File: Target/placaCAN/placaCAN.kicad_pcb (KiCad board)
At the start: 2 copper layers, 5 parts, among them J1 Can1, J2 Can2, j3 a PC

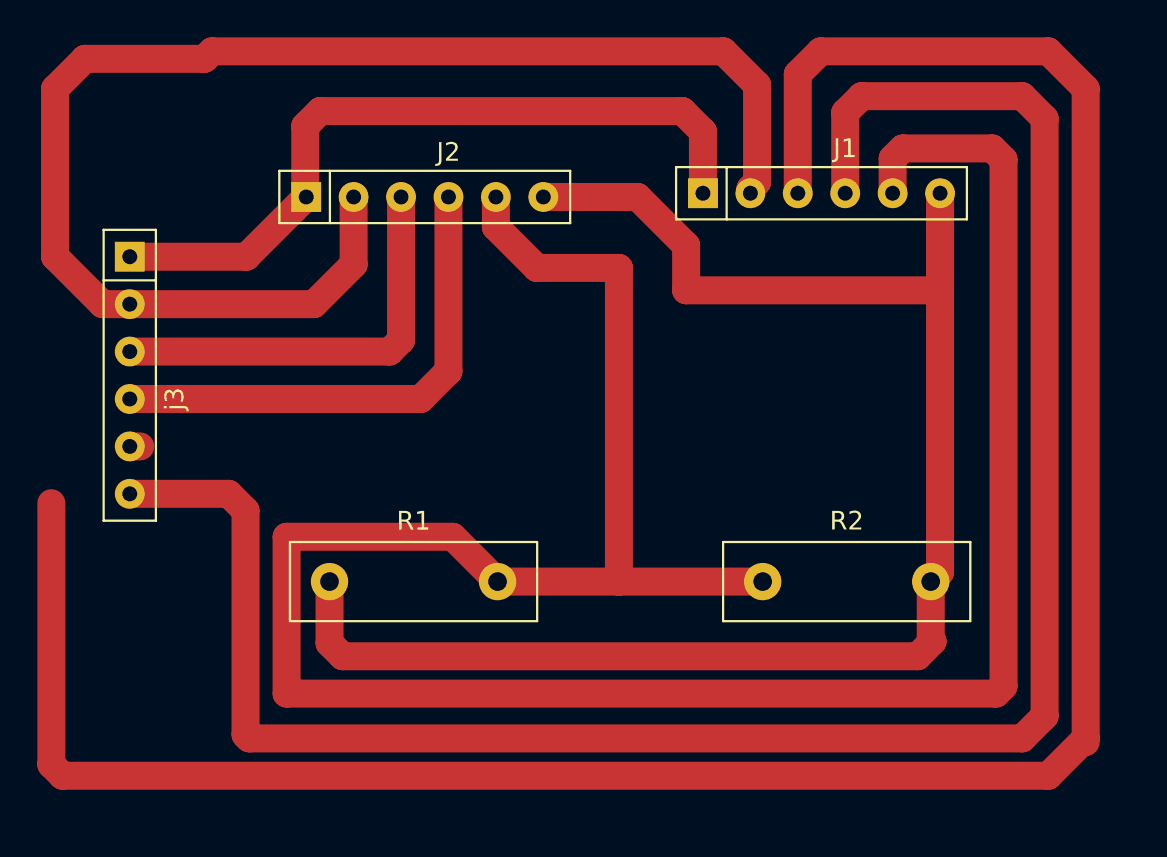
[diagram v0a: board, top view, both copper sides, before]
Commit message: actualizo
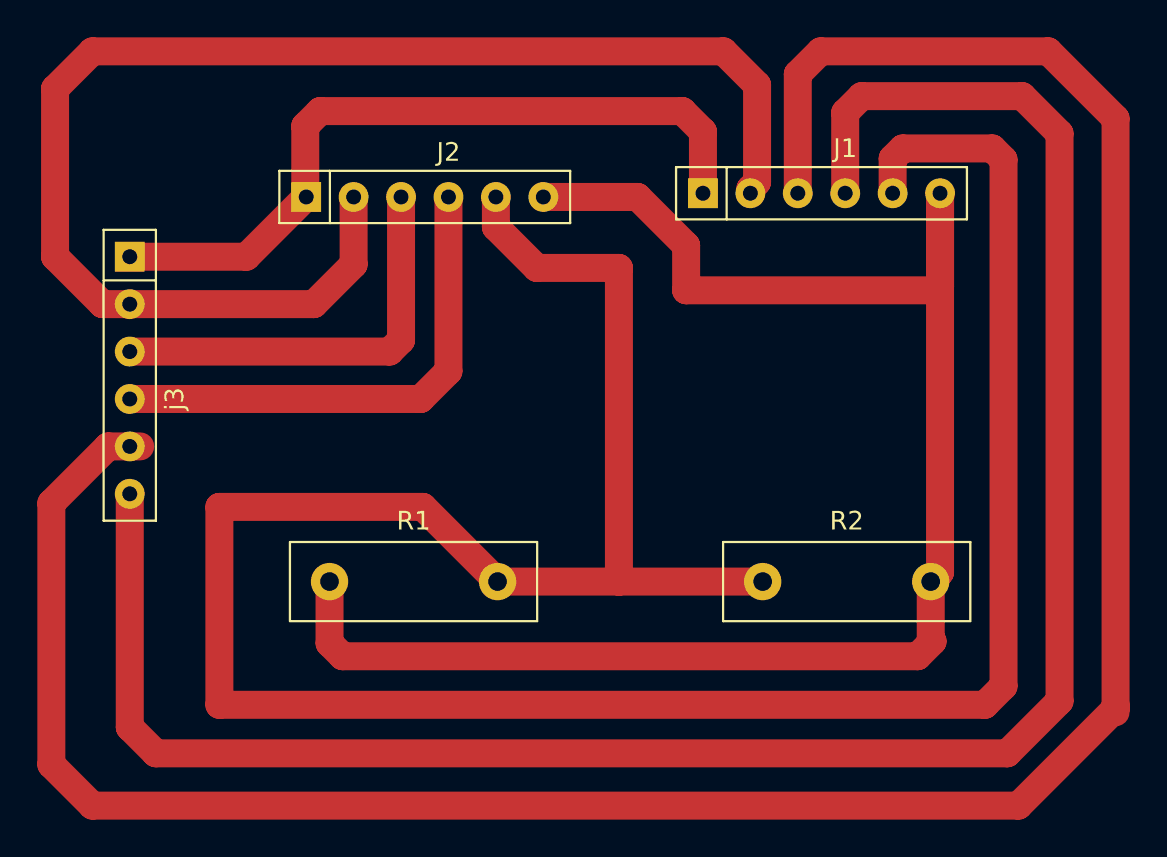
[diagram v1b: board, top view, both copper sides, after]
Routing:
- net Net-(J1-Pad5): track 135.8 -> 146.2 mm
- net Net-(J1-Pad3): track 129.2 -> 137.5 mm
- net Net-(J1-Pad4): track 109.8 -> 111.4 mm
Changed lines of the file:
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@@
   (segment (start 122.2 69.95) (end 122.25 70) (width 1.5) (layer "F.Cu") (net 1))
   (segment (start 124.79 73.61) (end 124.79 70) (width 1.5) (layer "F.Cu") (net 2))
-  (segment (start 117.2 62.2) (end 144.6 62.2) (width 1.5) (layer "F.Cu") (net 2))
-  (segment (start 146.4 69.2) (end 146.04 69.56) (width 1.5) (layer "F.Cu") (net 2))
+  (segment (start 144.6 62.2) (end 146.4 64) (width 1.5) (layer "F.Cu") (net 2))
   (segment (start 112.8 75.74) (end 111.34 75.74) (width 1.5) (layer "F.Cu") (net 2))
   (segment (start 122.66 75.74) (end 124.79 73.61) (width 1.5) (layer "F.Cu") (net 2))
   (segment (start 112.8 75.74) (end 122.66 75.74) (width 1.5) (layer "F.Cu") (net 2))
-  (segment (start 144.6 62.2) (end 146.4 64) (width 1.5) (layer "F.Cu") (net 2))
-  (segment (start 108.8 64.2) (end 110.4 62.6) (width 1.5) (layer "F.Cu") (net 2))
-  (segment (start 116.8 62.6) (end 117.2 62.2) (width 1.5) (layer "F.Cu") (net 2))
+  (segment (start 111.34 75.74) (end 108.8 73.2) (width 1.5) (layer "F.Cu") (net 2))
+  (segment (start 108.8 64.2) (end 110.8 62.2) (width 1.5) (layer "F.Cu") (net 2))
+  (segment (start 146.4 69.2) (end 146.04 69.56) (width 1.5) (layer "F.Cu") (net 2))
+  (segment (start 146.4 64) (end 146.4 69.2) (width 1.5) (layer "F.Cu") (net 2))
   (segment (start 108.8 73.2) (end 108.8 64.2) (width 1.5) (layer "F.Cu") (net 2))
-  (segment (start 111.34 75.74) (end 108.8 73.2) (width 1.5) (layer "F.Cu") (net 2))
-  (segment (start 146.4 64) (end 146.4 69.2) (width 1.5) (layer "F.Cu") (net 2))
   (segment (start 146.04 69.56) (end 146.04 69.8) (width 1.5) (layer "F.Cu") (net 2))
-  (segment (start 110.4 62.6) (end 116.8 62.6) (width 1.5) (layer "F.Cu") (net 2))
-  (segment (start 149.8 62.2) (end 162 62.2) (width 1.5) (layer "F.Cu") (net 3))
+  (segment (start 110.8 62.2) (end 144.6 62.2) (width 1.5) (layer "F.Cu") (net 2))
+  (segment (start 165.6 97.2) (end 165.6 97.4) (width 1.5) (layer "F.Cu") (net 3))
   (segment (start 148.58 63.42) (end 149.8 62.2) (width 1.5) (layer "F.Cu") (net 3))
   (segment (start 113.36 83.36) (end 112.8 83.36) (width 1.5) (layer "F.Cu") (net 3))
-  (segment (start 162 62.2) (end 164 64.2) (width 1.5) (layer "F.Cu") (net 3))
-  (segment (start 164 64.2) (end 164 99.2) (width 1.5) (layer "F.Cu") (net 3))
+  (segment (start 160.4 102.6) (end 110.8 102.6) (width 1.5) (layer "F.Cu") (net 3))
+  (segment (start 165.6 65.8) (end 165.6 97.6) (width 1.5) (layer "F.Cu") (net 3))
+  (segment (start 110.8 102.6) (end 108.6 100.4) (width 1.5) (layer "F.Cu") (net 3))
+  (segment (start 148.58 69.8) (end 148.58 63.42) (width 1.5) (layer "F.Cu") (net 3))
   (segment (start 108.6 100.4) (end 108.6 86.4) (width 1.5) (layer "F.Cu") (net 3))
-  (segment (start 164 99) (end 162 101) (width 1.5) (layer "F.Cu") (net 3))
-  (segment (start 109.2 101) (end 108.6 100.4) (width 1.5) (layer "F.Cu") (net 3))
-  (segment (start 162 101) (end 109.2 101) (width 1.5) (layer "F.Cu") (net 3))
-  (segment (start 148.58 69.8) (end 148.58 63.42) (width 1.5) (layer "F.Cu") (net 3))
-  (segment (start 118.1 85.9) (end 119 86.8) (width 1.5) (layer "F.Cu") (net 4))
-  (segment (start 161.8 97.8) (end 160.6 99) (width 1.5) (layer "F.Cu") (net 4))
-  (segment (start 160.6 99) (end 119.2 99) (width 1.5) (layer "F.Cu") (net 4))
+  (segment (start 111.64 83.36) (end 112.8 83.36) (width 1.5) (layer "F.Cu") (net 3))
+  (segment (start 165.6 97.4) (end 160.4 102.6) (width 1.5) (layer "F.Cu") (net 3))
+  (segment (start 108.6 86.4) (end 111.64 83.36) (width 1.5) (layer "F.Cu") (net 3))
+  (segment (start 149.8 62.2) (end 162 62.2) (width 1.5) (layer "F.Cu") (net 3))
+  (segment (start 162 62.2) (end 165.6 65.8) (width 1.5) (layer "F.Cu") (net 3))
+  (segment (start 162.6 97) (end 159.8 99.8) (width 1.5) (layer "F.Cu") (net 4))
+  (segment (start 114.2 99.8) (end 112.8 98.4) (width 1.5) (layer "F.Cu") (net 4))
+  (segment (start 152 64.6) (end 160.6 64.6) (width 1.5) (layer "F.Cu") (net 4))
+  (segment (start 160.6 64.6) (end 162.6 66.6) (width 1.5) (layer "F.Cu") (net 4))
   (segment (start 151.12 69.8) (end 151.12 65.48) (width 1.5) (layer "F.Cu") (net 4))
-  (segment (start 119.2 99) (end 119 98.8) (width 1.5) (layer "F.Cu") (net 4))
-  (segment (start 160.6 64.6) (end 161.8 65.8) (width 1.5) (layer "F.Cu") (net 4))
-  (segment (start 152 64.6) (end 160.6 64.6) (width 1.5) (layer "F.Cu") (net 4))
-  (segment (start 112.8 85.9) (end 118.1 85.9) (width 1.5) (layer "F.Cu") (net 4))
-  (segment (start 161.8 65.8) (end 161.8 97.8) (width 1.5) (layer "F.Cu") (net 4))
   (segment (start 151.12 65.48) (end 152 64.6) (width 1.5) (layer "F.Cu") (net 4))
-  (segment (start 119 98.8) (end 119 86.8) (width 1.5) (layer "F.Cu") (net 4))
+  (segment (start 159.8 99.8) (end 114.2 99.8) (width 1.5) (layer "F.Cu") (net 4))
+  (segment (start 112.8 98.4) (end 112.8 85.9) (width 1.5) (layer "F.Cu") (net 4))
+  (segment (start 162.6 66.6) (end 162.6 97) (width 1.5) (layer "F.Cu") (net 4))
+  (segment (start 159 67.4) (end 159.6 68) (width 1.5) (layer "F.Cu") (net 5))
+  (segment (start 159.6 96.2) (end 158.6 97.2) (width 1.5) (layer "F.Cu") (net 5))
   (segment (start 153.66 69.8) (end 153.66 67.94) (width 1.5) (layer "F.Cu") (net 5))
-  (segment (start 154.2 67.4) (end 159 67.4) (width 1.5) (layer "F.Cu") (net 5))
-  (segment (start 121.2 96.6) (end 121.2 88.2) (width 1.5) (layer "F.Cu") (net 5))
-  (segment (start 121.2 88.2) (end 130.1 88.2) (width 1.5) (layer "F.Cu") (net 5))
+  (segment (start 117.6 86.6) (end 128.5 86.6) (width 1.5) (layer "F.Cu") (net 5))
+  (segment (start 117.6 97.2) (end 117.6 86.6) (width 1.5) (layer "F.Cu") (net 5))
   (segment (start 134.6 73.8) (end 139 73.8) (width 1.5) (layer "F.Cu") (net 5))
-  (segment (start 130.1 88.2) (end 132.5 90.6) (width 1.5) (layer "F.Cu") (net 5))
+  (segment (start 128.5 86.6) (end 132.5 90.6) (width 1.5) (layer "F.Cu") (net 5))
+  (segment (start 139 90.6) (end 132.5 90.6) (width 1.5) (layer "F.Cu") (net 5))
   (segment (start 153.66 67.94) (end 154.2 67.4) (width 1.5) (layer "F.Cu") (net 5))
-  (segment (start 159 67.4) (end 159.6 68) (width 1.5) (layer "F.Cu") (net 5))
-  (segment (start 139 90.6) (end 132.5 90.6) (width 1.5) (layer "F.Cu") (net 5))
   (segment (start 159.6 68) (end 159.6 96.2) (width 1.5) (layer "F.Cu") (net 5))
-  (segment (start 159.2 96.6) (end 121.2 96.6) (width 1.5) (layer "F.Cu") (net 5))
   (segment (start 132.41 70) (end 132.41 71.61) (width 1.5) (layer "F.Cu") (net 5))
-  (segment (start 159.6 96.2) (end 159.2 96.6) (width 1.5) (layer "F.Cu") (net 5))
+  (segment (start 158.6 97.2) (end 117.6 97.2) (width 1.5) (layer "F.Cu") (net 5))
   (segment (start 139 73.8) (end 139 90.6) (width 1.5) (layer "F.Cu") (net 5))
   (segment (start 132.41 71.61) (end 134.6 73.8) (width 1.5) (layer "F.Cu") (net 5))
+  (segment (start 154.2 67.4) (end 159 67.4) (width 1.5) (layer "F.Cu") (net 5))
   (segment (start 146.7 90.6) (end 139 90.6) (width 1.5) (layer "F.Cu") (net 5))
   (segment (start 155 94.6) (end 155.8 93.8) (width 1.5) (layer "F.Cu") (net 6))
